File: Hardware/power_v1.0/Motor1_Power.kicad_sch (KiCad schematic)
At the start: 16 parts, among them J1 Conn_01x02, U1 MP2338GTL-Z

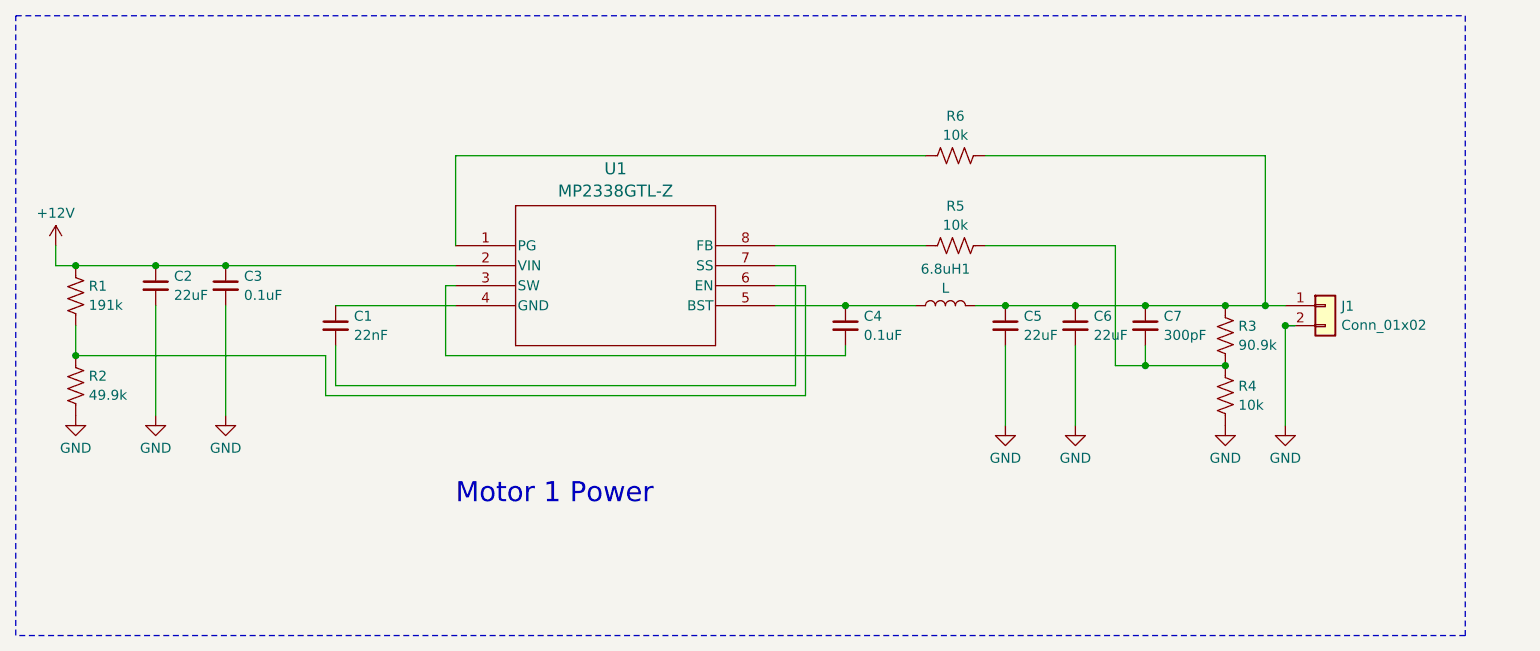
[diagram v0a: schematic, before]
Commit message: almost finished design of power board and working through design of brain board
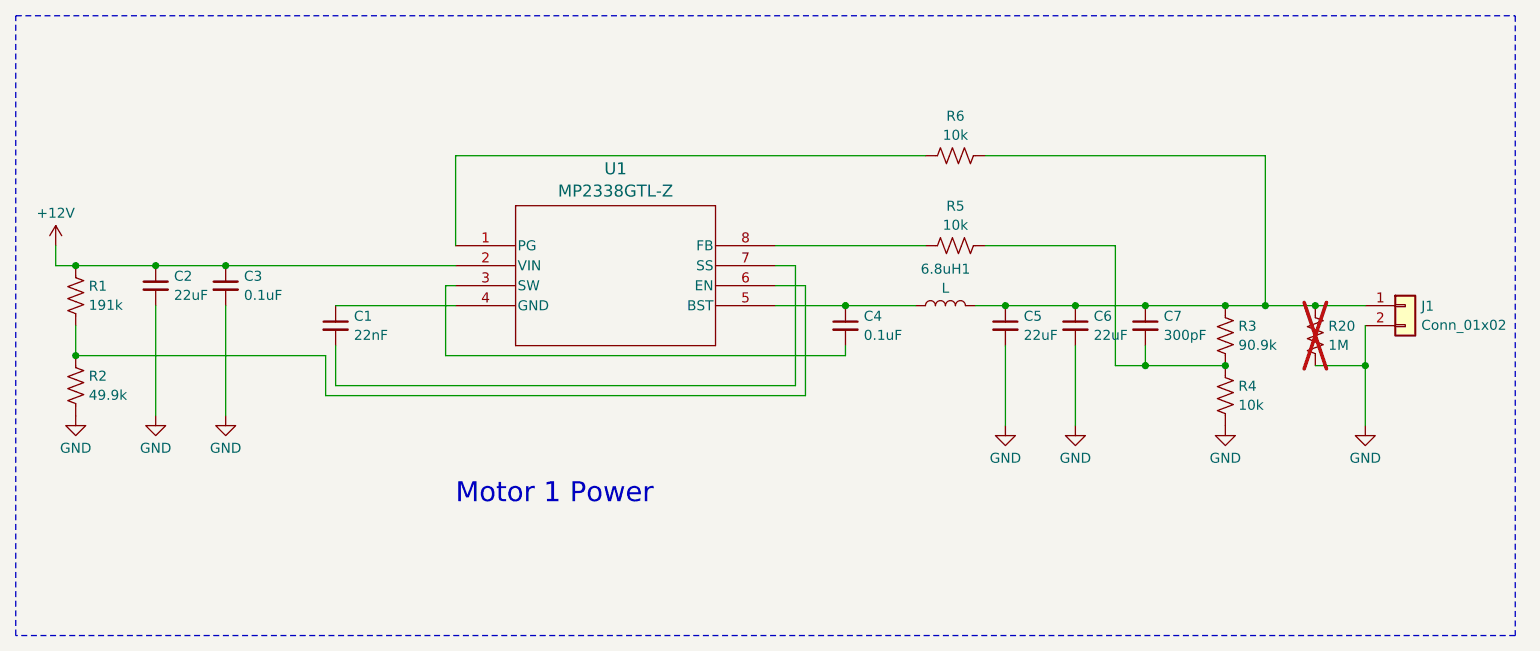
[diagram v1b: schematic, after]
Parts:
- added R20: 1M, symbol Device:R_US
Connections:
- net GND: now also R20.2
- net at 6.8uH1.2, C5.1, C6.1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: now also R20.1
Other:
- moved on the sheet: J1
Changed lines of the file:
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@@
   (junction (at 184.15 95.25) (diameter 0) (color 0 0 0 0)
   )
-  (junction (at 219.71 97.79) (diameter 0) (color 0 0 0 0)
-  )
   (junction (at 212.09 95.25) (diameter 0) (color 0 0 0 0)
   )
   (junction (at 66.04 90.17) (diameter 0) (color 0 0 0 0)
   )
+  (junction (at 229.87 102.87) (diameter 0) (color 0 0 0 0)
+  )
   (junction (at 85.09 90.17) (diameter 0) (color 0 0 0 0)
   )
@@
   (junction (at 212.09 102.87) (diameter 0) (color 0 0 0 0)
   )
+  (junction (at 223.52 95.25) (diameter 0) (color 0 0 0 0)
+  )
   (wire (pts (xy 212.09 95.25) (xy 217.17 95.25))
     (stroke (width 0) (type default))
@@
     (stroke (width 0) (type default))
   )
+  (wire (pts (xy 229.87 102.87) (xy 229.87 110.49))
+    (stroke (width 0) (type default))
+  )
   (wire (pts (xy 114.3 87.63) (xy 114.3 76.2))
     (stroke (width 0) (type default))
@@
     (stroke (width 0) (type default))
   )
+  (wire (pts (xy 223.52 95.25) (xy 229.87 95.25))
+    (stroke (width 0) (type default))
+  )
   (wire (pts (xy 158.75 106.68) (xy 158.75 92.71))
     (stroke (width 0) (type default))
   )
-  (wire (pts (xy 217.17 95.25) (xy 219.71 95.25))
-    (stroke (width 0) (type default))
-  )
-  (wire (pts (xy 219.71 97.79) (xy 220.98 97.79))
+  (wire (pts (xy 217.17 95.25) (xy 223.52 95.25))
     (stroke (width 0) (type default))
   )
@@
     (stroke (width 0) (type default))
   )
-  (wire (pts (xy 219.71 97.79) (xy 219.71 110.49))
+  (wire (pts (xy 229.87 97.79) (xy 229.87 102.87))
     (stroke (width 0) (type default))
   )
@@
     (stroke (width 0) (type default))
   )
+  (wire (pts (xy 223.52 102.87) (xy 229.87 102.87))
+    (stroke (width 0) (type default))
+  )
   (wire (pts (xy 157.48 105.41) (xy 157.48 90.17))
     (stroke (width 0) (type default))
@@
     (stroke (width 0) (type default))
   )
-  (rectangle (start 58.42 58.42) (end 242.57 137.16)
+  (rectangle (start 58.42 58.42) (end 248.92 137.16)
     (stroke (width 0) (type dash))
     (fill (type none))
@@
     )
   )
-  (symbol (lib_id "Connector_Generic:Conn_01x02") (at 224.79 95.25 0) (unit 1)
-    (in_bom yes) (on_board yes) (dnp no) (fields_autoplaced)
-    (property "Reference" "J1" (at 226.822 95.3079 0)
-      (effects (font (size 1.27 1.27)) (justify left))
-    )
-    (property "Value" "Conn_01x02" (at 226.822 97.7321 0)
-      (effects (font (size 1.27 1.27)) (justify left))
-    )
-    (property "Footprint" "" (at 224.79 95.25 0)
-      (effects (font (size 1.27 1.27)) hide)
-    )
-    (property "Datasheet" "~" (at 224.79 95.25 0)
+  (symbol (lib_id "Connector_Generic:Conn_01x02") (at 234.95 95.25 0) (unit 1)
+    (in_bom yes) (on_board yes) (dnp no) (fields_autoplaced)
+    (property "Reference" "J1" (at 236.982 95.3079 0)
+      (effects (font (size 1.27 1.27)) (justify left))
+    )
+    (property "Value" "Conn_01x02" (at 236.982 97.7321 0)
+      (effects (font (size 1.27 1.27)) (justify left))
+    )
+    (property "Footprint" "" (at 234.95 95.25 0)
+      (effects (font (size 1.27 1.27)) hide)
+    )
+    (property "Datasheet" "~" (at 234.95 95.25 0)
       (effects (font (size 1.27 1.27)) hide)
     )
@@
     )
   )
-  (symbol (lib_id "power:GND") (at 219.71 110.49 0) (unit 1)
-    (in_bom yes) (on_board yes) (dnp no) (fields_autoplaced)
-    (property "Reference" "#PWR09" (at 219.71 116.84 0)
-      (effects (font (size 1.27 1.27)) hide)
-    )
-    (property "Value" "GND" (at 219.71 114.6231 0)
-      (effects (font (size 1.27 1.27)))
-    )
-    (property "Footprint" "" (at 219.71 110.49 0)
-      (effects (font (size 1.27 1.27)) hide)
-    )
-    (property "Datasheet" "" (at 219.71 110.49 0)
+  (symbol (lib_id "power:GND") (at 229.87 110.49 0) (unit 1)
+    (in_bom yes) (on_board yes) (dnp no) (fields_autoplaced)
+    (property "Reference" "#PWR09" (at 229.87 116.84 0)
+      (effects (font (size 1.27 1.27)) hide)
+    )
+    (property "Value" "GND" (at 229.87 114.6231 0)
+      (effects (font (size 1.27 1.27)))
+    )
+    (property "Footprint" "" (at 229.87 110.49 0)
+      (effects (font (size 1.27 1.27)) hide)
+    )
+    (property "Datasheet" "" (at 229.87 110.49 0)
       (effects (font (size 1.27 1.27)) hide)
     )
@@
         )
       )
+    )
+  )
+  (symbol (lib_id "Device:R_US") (at 223.52 99.06 0) (unit 1)
+    (in_bom yes) (on_board yes) (dnp yes) (fields_autoplaced)
+    (property "Reference" "R20" (at 225.171 97.8479 0)
+      (effects (font (size 1.27 1.27)) (justify left))
+    )
+    (property "Value" "1M" (at 225.171 100.2721 0)
+      (effects (font (size 1.27 1.27)) (justify left))
+    )
+    (property "Footprint" "" (at 224.536 99.314 90)
+      (effects (font (size 1.27 1.27)) hide)
+    )
+    (property "Datasheet" "~" (at 223.52 99.06 0)
+      (effects (font (size 1.27 1.27)) hide)
+    )
+    (pin "1")
+    (pin "2")
+    (instances
+      (project "power_v1.0"
+        (path "/1e1b062d-fad0-427c-a622-c5b8a80b5268/746743d3-7add-4a0e-9b89-d67b4a6bc52a"
+          (reference "R20") (unit 1)
+        )
+      )
